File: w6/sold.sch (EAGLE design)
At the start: 35 parts, among them T1 50v 16A N-channel, U1 AD8615AUJ, U2 AD8615AUJ

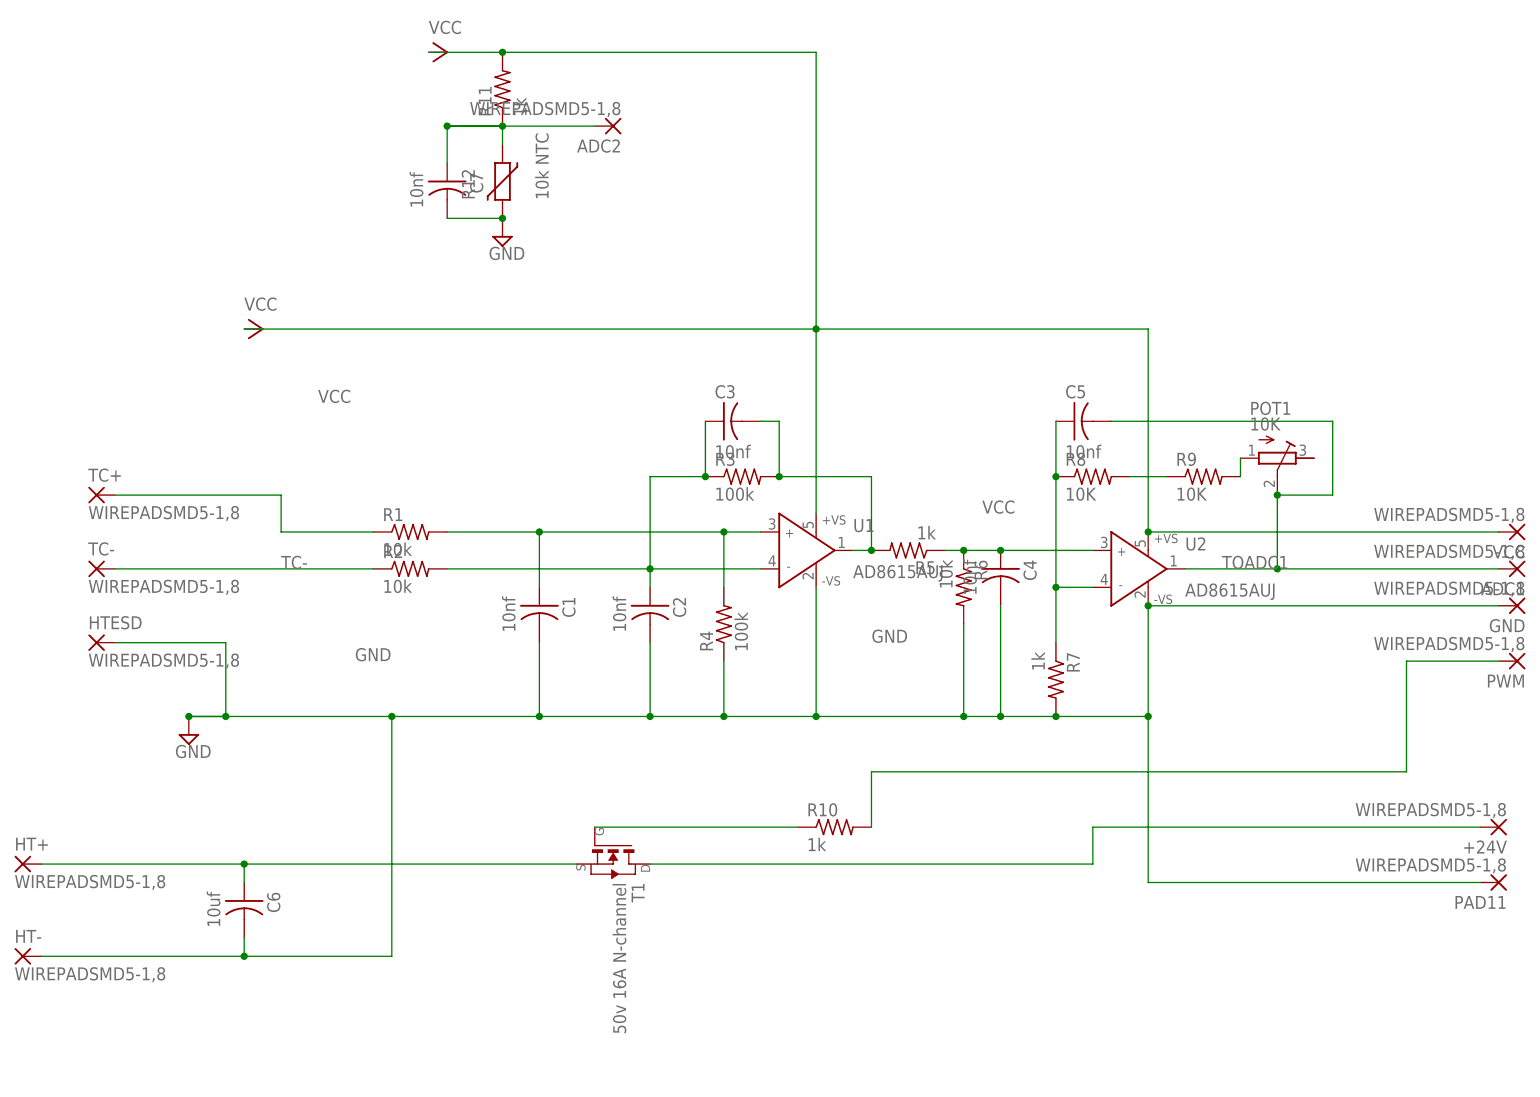
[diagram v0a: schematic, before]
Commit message: shopbot done and many other typos and w6 8 9 10 11 12 proof
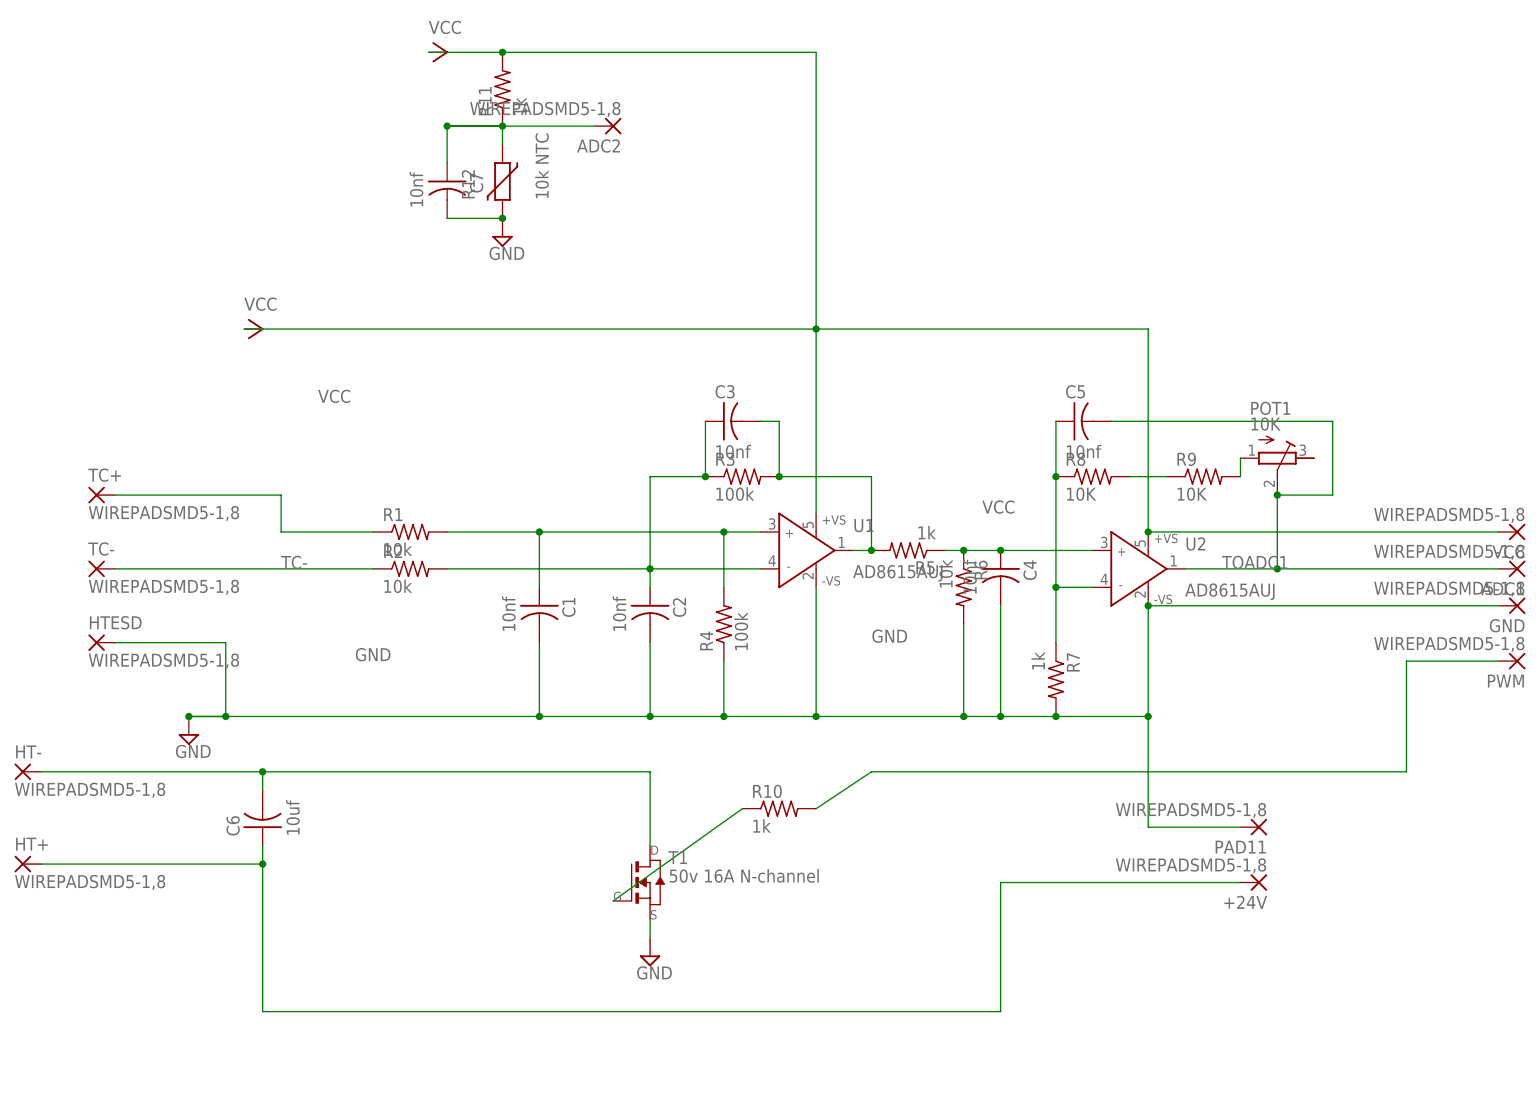
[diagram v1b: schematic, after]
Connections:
- removed net N$9: C6.1, HT+.P, T1.S
- new net N$15: C6.2, HT-.P, T1.D
- net GND: now also T1.S; no longer C6.2, HT-.P
- net N$14: now also C6.1, HT+.P; no longer T1.D
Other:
- moved on the sheet: +24V, C6, HT-, PAD11, R10, T1
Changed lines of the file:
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@@
 <?xml version="1.0" encoding="utf-8"?>
 <!DOCTYPE eagle SYSTEM "eagle.dtd">
-<eagle version="7.4.0">
+<eagle version="7.6.0">
 <drawing>
 <settings>
@@
 <part name="P+2" library="supply1" deviceset="VCC" device=""/>
 <part name="ADC2" library="wirepad" deviceset="WIREPAD" device="SMD5-1,8"/>
+<part name="SUPPLY3" library="supply2" deviceset="GND" device=""/>
 </parts>
 <sheets>
@@
 <instance part="TC-" gate="G$1" x="-99.06" y="22.86"/>
 <instance part="HT+" gate="G$1" x="-109.22" y="-17.78"/>
-<instance part="HT-" gate="G$1" x="-109.22" y="-30.48"/>
-<instance part="+24V" gate="G$1" x="93.98" y="-12.7" rot="R180"/>
-<instance part="PAD11" gate="G$1" x="93.98" y="-20.32" rot="R180"/>
-<instance part="R10" gate="G$1" x="2.54" y="-12.7"/>
-<instance part="C6" gate="G$1" x="-78.74" y="-22.86" rot="R270"/>
-<instance part="T1" gate="A" x="-27.94" y="-17.78" rot="R270"/>
+<instance part="HT-" gate="G$1" x="-109.22" y="-5.08"/>
+<instance part="+24V" gate="G$1" x="60.96" y="-20.32" rot="R180"/>
+<instance part="PAD11" gate="G$1" x="60.96" y="-12.7" rot="R180"/>
+<instance part="R10" gate="G$1" x="-5.08" y="-10.16"/>
+<instance part="C6" gate="G$1" x="-76.2" y="-12.7" rot="R90"/>
+<instance part="T1" gate="A" x="-22.86" y="-20.32"/>
 <instance part="SUPPLY1" gate="GND" x="-86.36" y="0"/>
 <instance part="C7" gate="G$1" x="-50.8" y="76.2" rot="R270"/>
@@
 <instance part="P+2" gate="VCC" x="-50.8" y="93.98" rot="R270"/>
 <instance part="ADC2" gate="G$1" x="-27.94" y="83.82" rot="R180"/>
+<instance part="SUPPLY3" gate="GND" x="-22.86" y="-30.48"/>
 </instances>
 <busses>
@@
 <junction x="0" y="2.54"/>
 <wire x1="-81.28" y1="2.54" x2="-86.36" y2="2.54" width="0.1524" layer="91"/>
-<wire x1="-86.36" y1="2.54" x2="-58.42" y2="2.54" width="0.1524" layer="91"/>
-<wire x1="-58.42" y1="2.54" x2="-38.1" y2="2.54" width="0.1524" layer="91"/>
+<wire x1="-86.36" y1="2.54" x2="-38.1" y2="2.54" width="0.1524" layer="91"/>
 <wire x1="-38.1" y1="2.54" x2="-22.86" y2="2.54" width="0.1524" layer="91"/>
 <wire x1="-22.86" y1="2.54" x2="-12.7" y2="2.54" width="0.1524" layer="91"/>
@@
 <pinref part="GND" gate="G$1" pin="P"/>
 <pinref part="PAD11" gate="G$1" pin="P"/>
-<wire x1="91.44" y1="-20.32" x2="45.72" y2="-20.32" width="0.1524" layer="91"/>
-<wire x1="45.72" y1="-20.32" x2="45.72" y2="2.54" width="0.1524" layer="91"/>
+<wire x1="58.42" y1="-12.7" x2="45.72" y2="-12.7" width="0.1524" layer="91"/>
+<wire x1="45.72" y1="-12.7" x2="45.72" y2="2.54" width="0.1524" layer="91"/>
 <junction x="45.72" y="2.54"/>
-<pinref part="HT-" gate="G$1" pin="P"/>
-<wire x1="-106.68" y1="-30.48" x2="-78.74" y2="-30.48" width="0.1524" layer="91"/>
-<wire x1="-78.74" y1="-30.48" x2="-58.42" y2="-30.48" width="0.1524" layer="91"/>
-<wire x1="-58.42" y1="-30.48" x2="-58.42" y2="2.54" width="0.1524" layer="91"/>
-<junction x="-58.42" y="2.54"/>
-<pinref part="C6" gate="G$1" pin="2"/>
-<wire x1="-78.74" y1="-27.94" x2="-78.74" y2="-30.48" width="0.1524" layer="91"/>
-<junction x="-78.74" y="-30.48"/>
 <pinref part="SUPPLY1" gate="GND" pin="GND"/>
 <junction x="-86.36" y="2.54"/>
@@
 <junction x="-43.18" y="71.12"/>
 </segment>
+<segment>
+<pinref part="T1" gate="A" pin="S"/>
+<pinref part="SUPPLY3" gate="GND" pin="GND"/>
+<wire x1="-22.86" y1="-25.4" x2="-22.86" y2="-27.94" width="0.1524" layer="91"/>
+</segment>
 </net>
 <net name="N$5" class="0">
@@
 <pinref part="R10" gate="G$1" pin="1"/>
 <pinref part="T1" gate="A" pin="G"/>
-<wire x1="-2.54" y1="-12.7" x2="-30.48" y2="-12.7" width="0.1524" layer="91"/>
+<wire x1="-10.16" y1="-10.16" x2="-27.94" y2="-22.86" width="0.1524" layer="91"/>
 </segment>
 </net>
@@
 <pinref part="R10" gate="G$1" pin="2"/>
 <wire x1="81.28" y1="-5.08" x2="7.62" y2="-5.08" width="0.1524" layer="91"/>
-<wire x1="7.62" y1="-5.08" x2="7.62" y2="-12.7" width="0.1524" layer="91"/>
+<wire x1="7.62" y1="-5.08" x2="0" y2="-10.16" width="0.1524" layer="91"/>
 </segment>
 </net>
 <net name="N$14" class="0">
 <segment>
-<wire x1="38.1" y1="-17.78" x2="38.1" y2="-12.7" width="0.1524" layer="91"/>
 <pinref part="+24V" gate="G$1" pin="P"/>
-<wire x1="38.1" y1="-12.7" x2="91.44" y2="-12.7" width="0.1524" layer="91"/>
-<pinref part="T1" gate="A" pin="D"/>
-<wire x1="-22.86" y1="-17.78" x2="38.1" y2="-17.78" width="0.1524" layer="91"/>
-</segment>
-</net>
-<net name="N$9" class="0">
-<segment>
+<wire x1="25.4" y1="-20.32" x2="58.42" y2="-20.32" width="0.1524" layer="91"/>
+<wire x1="25.4" y1="-20.32" x2="25.4" y2="-38.1" width="0.1524" layer="91"/>
 <pinref part="HT+" gate="G$1" pin="P"/>
-<pinref part="T1" gate="A" pin="S"/>
-<wire x1="-106.68" y1="-17.78" x2="-78.74" y2="-17.78" width="0.1524" layer="91"/>
+<wire x1="-106.68" y1="-17.78" x2="-76.2" y2="-17.78" width="0.1524" layer="91"/>
 <pinref part="C6" gate="G$1" pin="1"/>
-<wire x1="-78.74" y1="-17.78" x2="-33.02" y2="-17.78" width="0.1524" layer="91"/>
-<wire x1="-78.74" y1="-17.78" x2="-78.74" y2="-20.32" width="0.1524" layer="91"/>
-<junction x="-78.74" y="-17.78"/>
+<wire x1="-76.2" y1="-17.78" x2="-76.2" y2="-15.24" width="0.1524" layer="91"/>
+<wire x1="25.4" y1="-38.1" x2="-76.2" y2="-38.1" width="0.1524" layer="91"/>
+<wire x1="-76.2" y1="-38.1" x2="-76.2" y2="-17.78" width="0.1524" layer="91"/>
+<junction x="-76.2" y="-17.78"/>
 </segment>
 </net>
@@
 </segment>
 </net>
+<net name="N$15" class="0">
+<segment>
+<pinref part="HT-" gate="G$1" pin="P"/>
+<wire x1="-106.68" y1="-5.08" x2="-76.2" y2="-5.08" width="0.1524" layer="91"/>
+<pinref part="C6" gate="G$1" pin="2"/>
+<wire x1="-76.2" y1="-7.62" x2="-76.2" y2="-5.08" width="0.1524" layer="91"/>
+<junction x="-76.2" y="-5.08"/>
+<pinref part="T1" gate="A" pin="D"/>
+<wire x1="-76.2" y1="-5.08" x2="-22.86" y2="-5.08" width="0.1524" layer="91"/>
+<wire x1="-22.86" y1="-5.08" x2="-22.86" y2="-15.24" width="0.1524" layer="91"/>
+</segment>
+</net>
